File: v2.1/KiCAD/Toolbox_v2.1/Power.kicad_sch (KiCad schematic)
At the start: 64 parts, among them J1 POWER, U1 TL074, U10 TL074, U11 TL074, U12 TL074, U13 CJ431, U14 CJ431, U15 CJ431, U2 TL074, U3 TL074, U4 TL074, U5 TL074, U6 TL074, U7 TL074, U8 TL074, U9 TL074

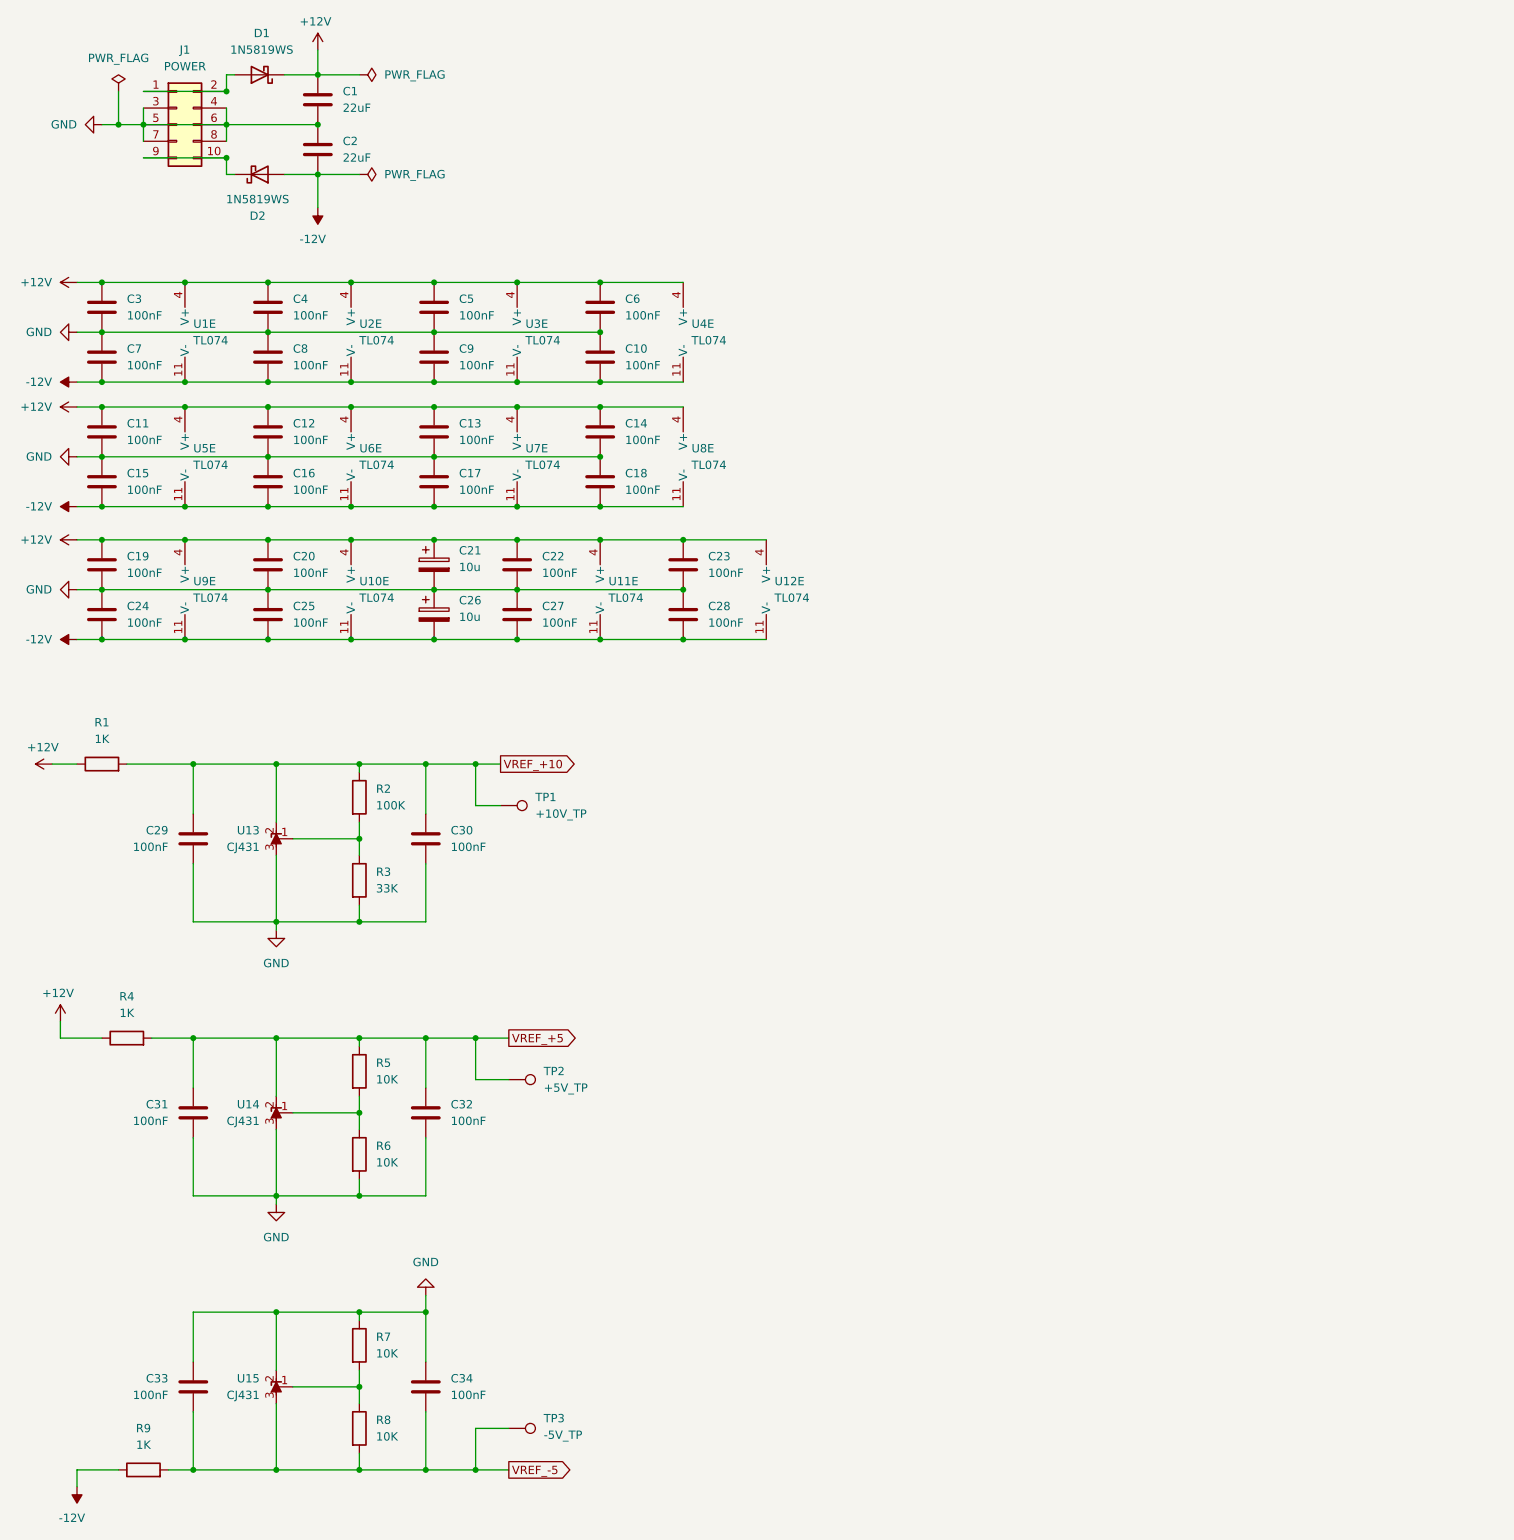
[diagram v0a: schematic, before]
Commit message: v2.1 Update
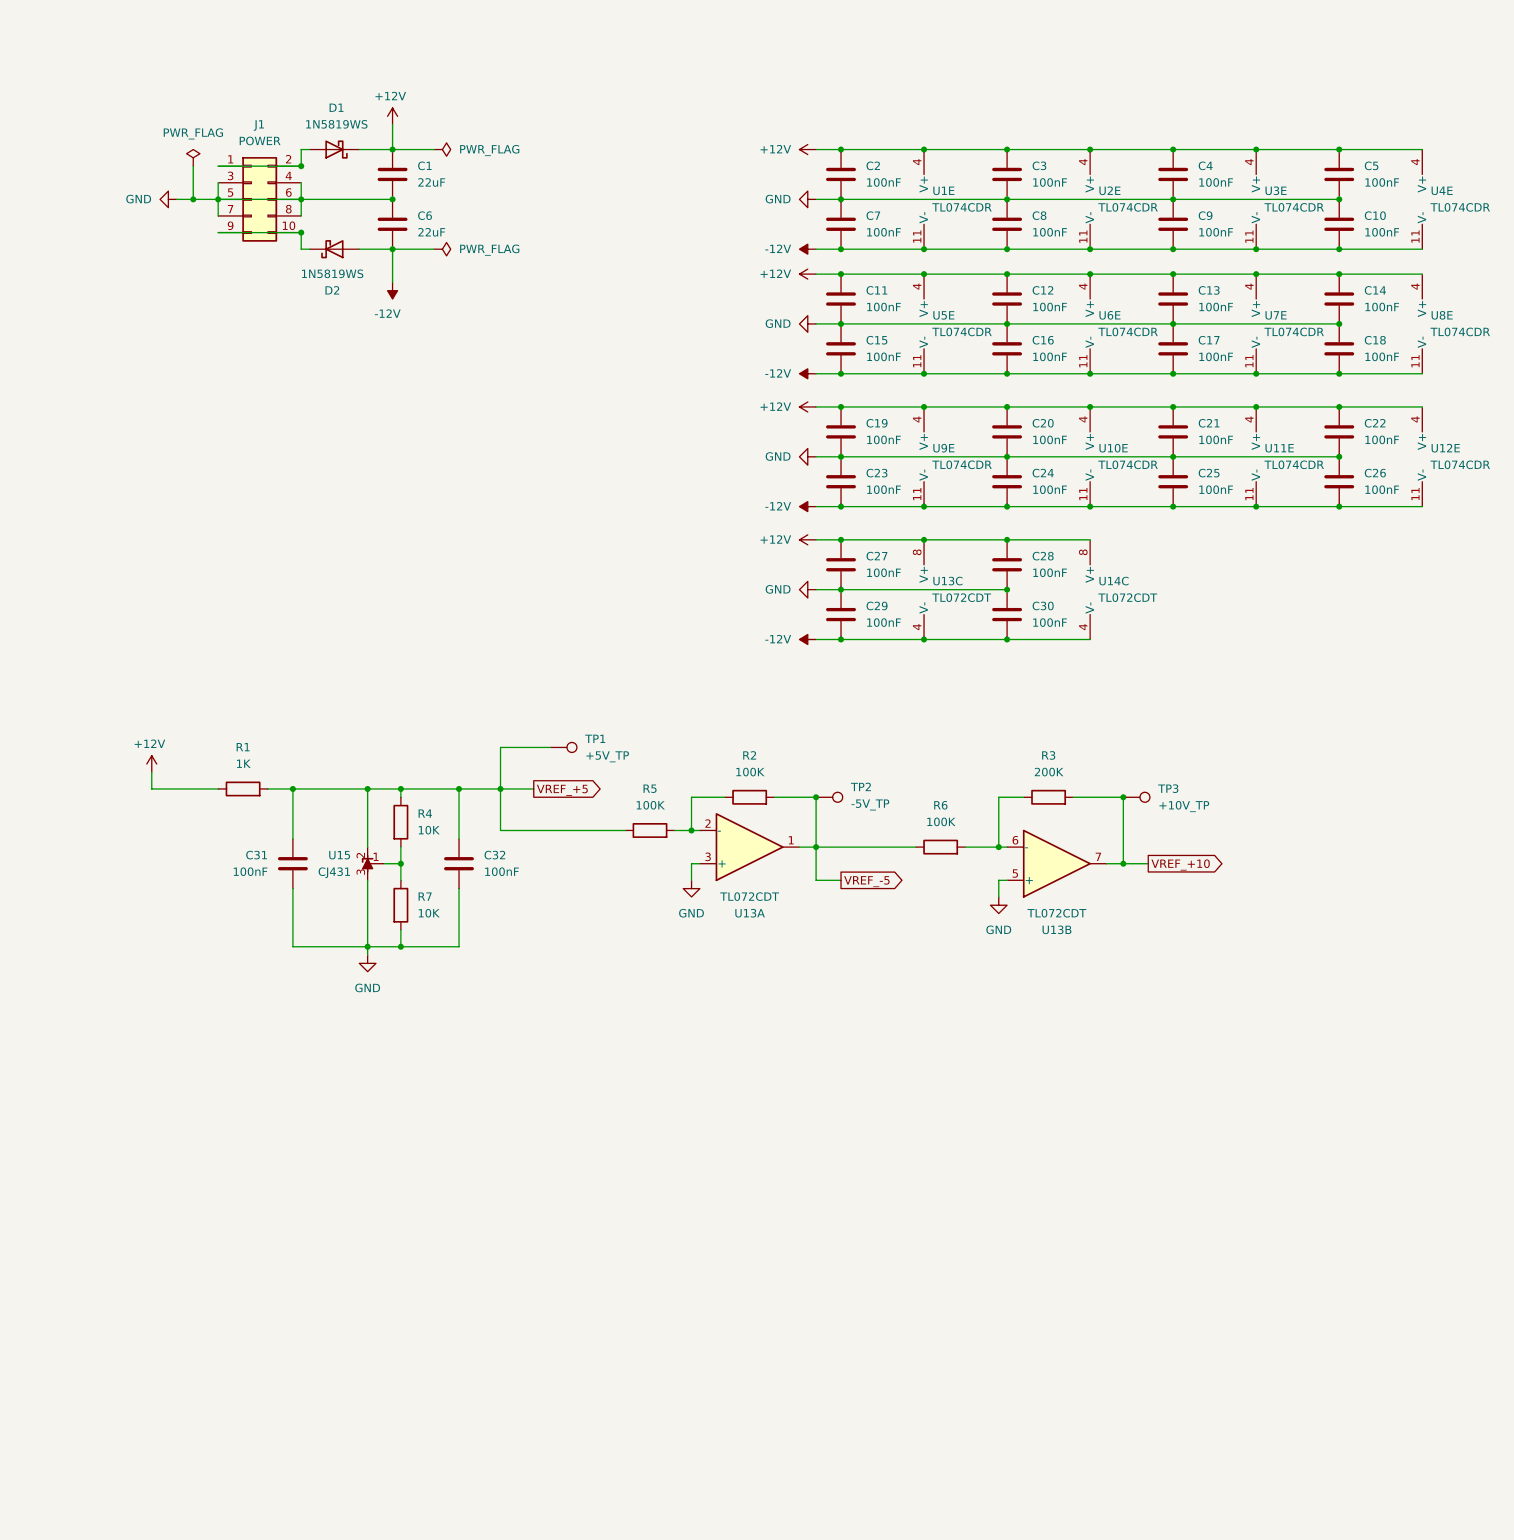
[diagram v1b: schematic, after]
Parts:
- removed C21, C26: 10u, Capacitor_Tantalum_SMD:CP_EIA-3216-18_Kemet-A, symbol Device:C_Polarized
- removed C33, C34, C6: 100nF, Capacitor_SMD:C_0402_1005Metric, symbol Device:C
- removed R1, R9: 1K, Resistor_SMD:R_0402_1005Metric, symbol Device:R
- removed R8: 10K, Resistor_SMD:R_0402_1005Metric, symbol Device:R
- removed U13, U15: CJ431, Package_TO_SOT_SMD:SOT-23, symbol kat_eurorack:CJ431
- added C21, C26, C3: 100nF, Capacitor_SMD:C_0603_1608Metric, symbol Device:C
- added R5: 100K, Resistor_SMD:R_0603_1608Metric, symbol Device:R
- added U13, U14: TL072CDT, Package_SO:SOIC-8_3.9x4.9mm_P1.27mm, symbol Amplifier_Operational:TL072
- C10, C11, C12, C13, C14, C15, C16, C17, C18, C19, C20, C22, C23, C24, C25, C27, C28, C29, C30, C31, C32, C4, C5, C7, C8, C9: footprint Capacitor_SMD:C_0402_1005Metric -> Capacitor_SMD:C_0603_1608Metric; LCSC C1525 -> C14663
- C2: renamed from C3; footprint Capacitor_SMD:C_0402_1005Metric -> Capacitor_SMD:C_0603_1608Metric; LCSC C1525 -> C14663
- R1: renamed from R4; footprint Resistor_SMD:R_0402_1005Metric -> Resistor_SMD:R_0603_1608Metric; LCSC C11702 -> C21190
- R2: footprint Resistor_SMD:R_0402_1005Metric -> Resistor_SMD:R_0603_1608Metric; LCSC C25741 -> C25803
- R3: value 33K -> 200K; footprint Resistor_SMD:R_0402_1005Metric -> Resistor_SMD:R_0603_1608Metric; LCSC C25779 -> C25811
- R4: renamed from R5; footprint Resistor_SMD:R_0402_1005Metric -> Resistor_SMD:R_0603_1608Metric; LCSC C25744 -> C25804
- R6: value 10K -> 100K; footprint Resistor_SMD:R_0402_1005Metric -> Resistor_SMD:R_0603_1608Metric; LCSC C25744 -> C25803
- R7: footprint Resistor_SMD:R_0402_1005Metric -> Resistor_SMD:R_0603_1608Metric; LCSC C25744 -> C25804
- U1, U10, U11, U12, U2, U3, U4, U6, U9: value TL074 -> TL074CDR; footprint Package_SO:TSSOP-14_4.4x5mm_P0.65mm -> Package_SO:SOIC-14_3.9x8.7mm_P1.27mm; LCSC C4370424 -> C12594
- U5, U7, U8: value TL074 -> TL074CDR; footprint Package_SO:TSSOP-14_4.4x5mm_P0.65mm -> Package_SO:SOIC-14_3.9x8.7mm_P1.27mm; LCSC (none) -> C12594
- renumbered C2 to C6, TP2 to TP1, TP3 to TP2, TP1 to TP3, U14 to U15
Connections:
- net +12V: now also C27.1, C28.1, C21.1, C3.1, U13.8 (V+), U14.8 (V+); no longer C23.1
- net -12V: now also C23.2, C29.2, C30.2, C26.2, U13.4 (V-), U14.4 (V-); no longer C27.2, C28.2
- net GND: now also C23.1, C27.2, C28.2, C29.1, C30.1, R7.2, C21.2, C26.1, C3.2, U13.3 (+), U13.5 (+); no longer C23.2, C27.1, C28.1, C29.2, C30.2, R3.2, R6.2, R7.1
- net VREF_+10: now also R3.2, U13.7; no longer C29.1, C30.1, R2.1
- net VREF_+5: now also R5.1
- net VREF_-5: now also R2.2, R6.1, U13.1
- net at R4.2, U15.1 (REF): now also R7.1; no longer R6.1
- net at R3.1: now also R6.2, U13.6 (-); no longer R2.2
- new net: R2.1, R5.2, U13.2 (-)
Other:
- moved on the sheet: C1, C2, C6, D1, D2, J1, R1, R4, TP1, TP2, TP3, U10E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
